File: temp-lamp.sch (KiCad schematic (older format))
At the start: 28 parts, among them P1 USB_5PIN_SHELL, P2 CONN_01X05, P3 CONN_01X08, P4 LED_1, P5 CONN_01X04, SW1 ON/OFF, SW2 RESET, SW3 PGM, U1 MCP73831, U2 ESP-12E, U3 SPX3819M5-3.3, U4 BME280

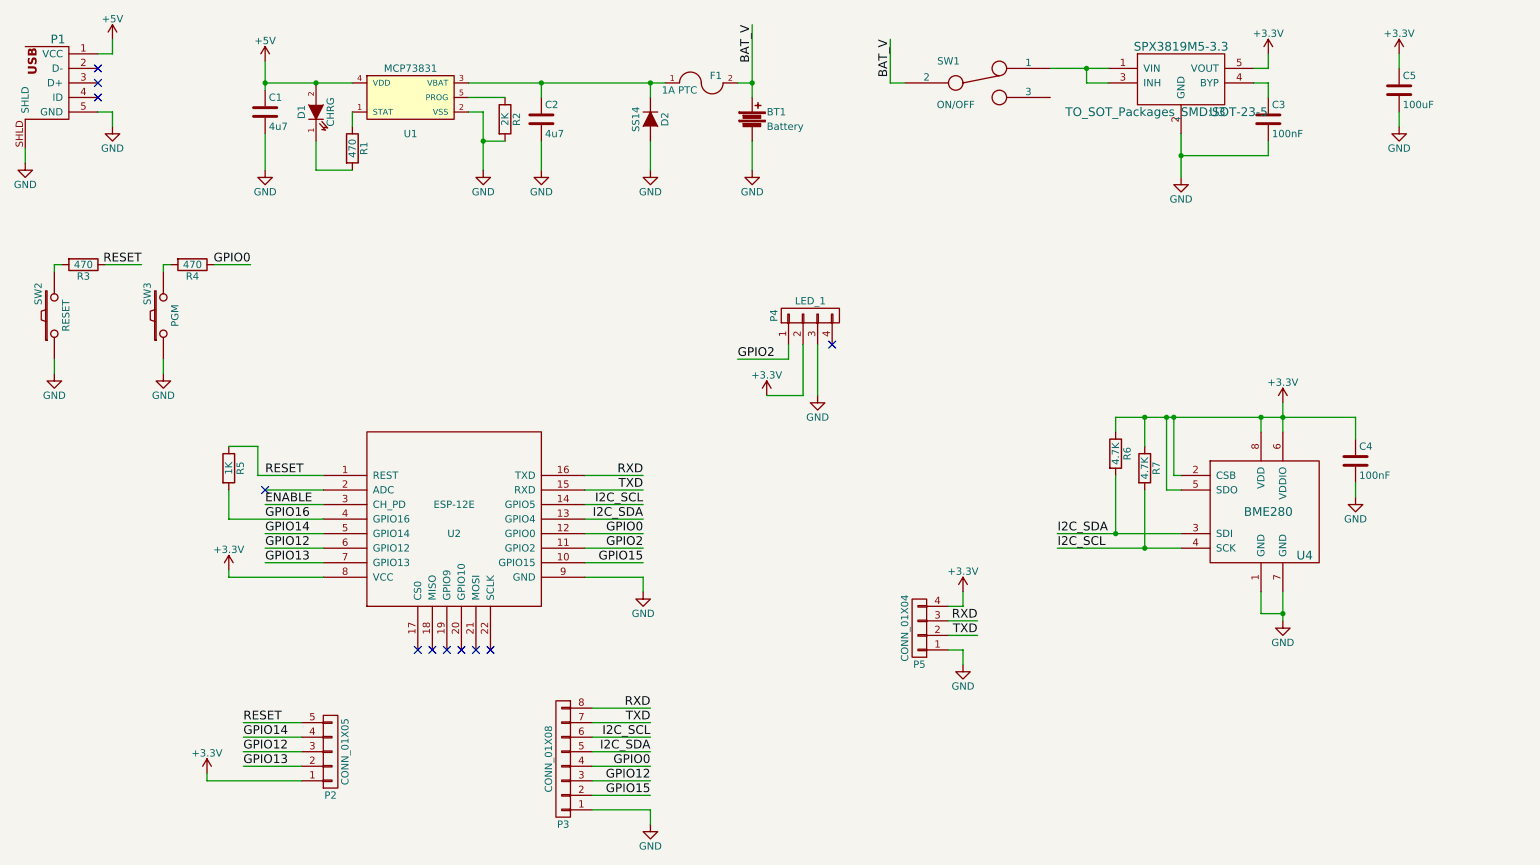
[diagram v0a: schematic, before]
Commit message: Updated pcb.
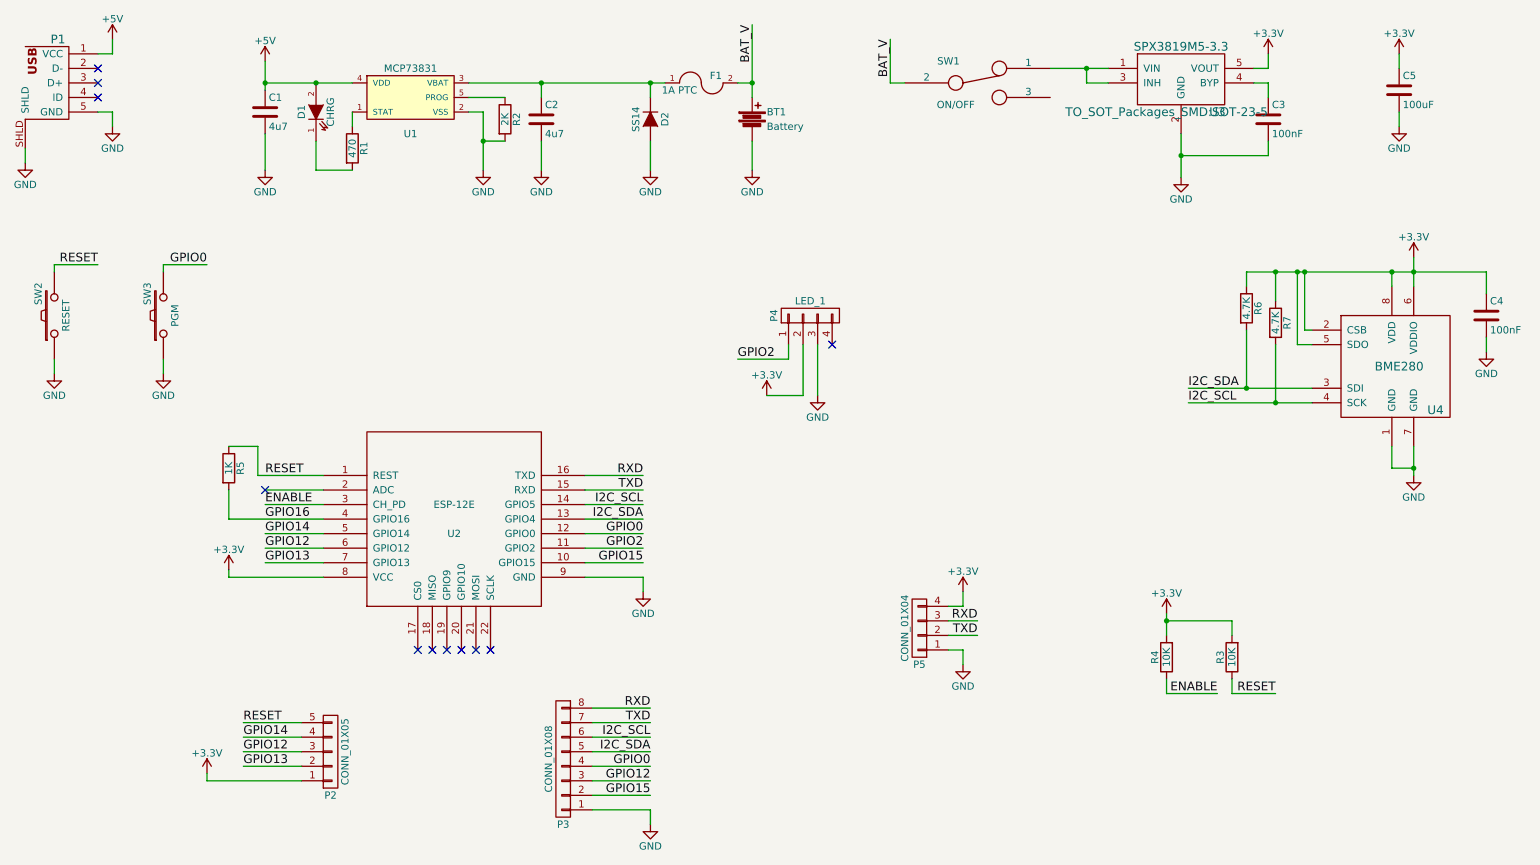
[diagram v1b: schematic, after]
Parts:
- C5: footprint Capacitors_SMD:C_0805_HandSoldering -> Capacitors_SMD:C_1206_HandSoldering
- R3, R4: value 470 -> 10K
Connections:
- net +3V3: now also R3.2, R4.2
- net ENABLE: now also R4.1
- net GPIO0: now also SW3.2; no longer R4.1
- net RESET: now also SW2.2
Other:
- moved on the sheet: C4, R3, R4, R6, R7, U4
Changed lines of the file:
@@
 LIBS:spx3819m5-3
 LIBS:ESP8266
-LIBS:temperature-lamp-cache
+LIBS:temp-lamp-cache
 EELAYER 25 0
 EELAYER END
@@
 	1    0    0    -1
 $EndComp
-$Comp
-L D D2
-U 1 1 5880BBE5
-P 5050 1550
-F 0 "D2" H 5050 1650 50  0000 C CNN
-F 1 "SS14" H 5050 1450 50  0000 C CNN
-F 2 "libs:DIODE_SMA" H 5050 1550 50  0001 C CNN
-F 3 "" H 5050 1550 50  0000 C CNN
-	1    5050 1550
-	0    1    1    0
-$EndComp
 Text Label 5750 900  3    60   ~ 0
 BAT_V
@@
 L BME280 U4
 U 1 1 5880DD6B
-P 9300 4250
-F 0 "U4" H 9550 3950 60  0000 C CNN
-F 1 "BME280" H 9300 4250 60  0000 C CNN
-F 2 "libs:BME280" H 9300 4250 60  0001 C CNN
-F 3 "" H 9300 4250 60  0000 C CNN
-	1    9300 4250
-	1    0    0    -1
-$EndComp
-Wire Wire Line
-	9250 4800 9250 4950
-Wire Wire Line
-	9250 4950 9400 4950
-Wire Wire Line
-	9400 4800 9400 5000
-Connection ~ 9400 4950
+P 10200 3250
+F 0 "U4" H 10450 2950 60  0000 C CNN
+F 1 "BME280" H 10200 3250 60  0000 C CNN
+F 2 "libs:BME280" H 10200 3250 60  0001 C CNN
+F 3 "" H 10200 3250 60  0000 C CNN
+	1    10200 3250
+	1    0    0    -1
+$EndComp
+Wire Wire Line
+	10150 3800 10150 3950
+Wire Wire Line
+	10150 3950 10300 3950
+Wire Wire Line
+	10300 3800 10300 4000
+Connection ~ 10300 3950
 $Comp
 L GND #PWR012
 U 1 1 5880E41C
-P 9400 5000
-F 0 "#PWR012" H 9400 4750 50  0001 C CNN
-F 1 "GND" H 9400 4850 50  0000 C CNN
-F 2 "" H 9400 5000 50  0000 C CNN
-F 3 "" H 9400 5000 50  0000 C CNN
-	1    9400 5000
+P 10300 4000
+F 0 "#PWR012" H 10300 3750 50  0001 C CNN
+F 1 "GND" H 10300 3850 50  0000 C CNN
+F 2 "" H 10300 4000 50  0000 C CNN
+F 3 "" H 10300 4000 50  0000 C CNN
+	1    10300 4000
 	1    0    0    -1
 $EndComp
@@
 L C C4
 U 1 1 5880E8AA
-P 9900 3900
-F 0 "C4" H 9925 4000 50  0000 L CNN
-F 1 "100nF" H 9925 3800 50  0000 L CNN
-F 2 "Capacitors_SMD:C_0603_HandSoldering" H 9938 3750 50  0001 C CNN
-F 3 "" H 9900 3900 50  0000 C CNN
-	1    9900 3900
+P 10800 2900
+F 0 "C4" H 10825 3000 50  0000 L CNN
+F 1 "100nF" H 10825 2800 50  0000 L CNN
+F 2 "Capacitors_SMD:C_0603_HandSoldering" H 10838 2750 50  0001 C CNN
+F 3 "" H 10800 2900 50  0000 C CNN
+	1    10800 2900
 	1    0    0    -1
 $EndComp
@@
 L GND #PWR013
 U 1 1 5880E9DC
-P 9900 4150
-F 0 "#PWR013" H 9900 3900 50  0001 C CNN
-F 1 "GND" H 9900 4000 50  0000 C CNN
-F 2 "" H 9900 4150 50  0000 C CNN
-F 3 "" H 9900 4150 50  0000 C CNN
-	1    9900 4150
-	1    0    0    -1
-$EndComp
-Wire Wire Line
-	9900 4150 9900 4050
+P 10800 3150
+F 0 "#PWR013" H 10800 2900 50  0001 C CNN
+F 1 "GND" H 10800 3000 50  0000 C CNN
+F 2 "" H 10800 3150 50  0000 C CNN
+F 3 "" H 10800 3150 50  0000 C CNN
+	1    10800 3150
+	1    0    0    -1
+$EndComp
+Wire Wire Line
+	10800 3150 10800 3050
 $Comp
 L +3.3V #PWR014
 U 1 1 5880EC60
-P 9400 3500
-F 0 "#PWR014" H 9400 3350 50  0001 C CNN
-F 1 "+3.3V" H 9400 3640 50  0000 C CNN
-F 2 "" H 9400 3500 50  0000 C CNN
-F 3 "" H 9400 3500 50  0000 C CNN
-	1    9400 3500
-	1    0    0    -1
-$EndComp
-Wire Wire Line
-	9900 3600 9900 3750
-Wire Wire Line
-	8250 3600 9900 3600
-Wire Wire Line
-	9400 3500 9400 3700
-Connection ~ 9400 3600
-Wire Wire Line
-	9250 3700 9250 3600
-Wire Wire Line
-	8700 4000 8650 4000
-Wire Wire Line
-	8650 4000 8650 3600
-Connection ~ 9250 3600
-Wire Wire Line
-	8700 4100 8600 4100
-Wire Wire Line
-	8600 4100 8600 3600
-Connection ~ 8650 3600
-Text Label 7850 4400 0    60   ~ 0
+P 10300 2500
+F 0 "#PWR014" H 10300 2350 50  0001 C CNN
+F 1 "+3.3V" H 10300 2640 50  0000 C CNN
+F 2 "" H 10300 2500 50  0000 C CNN
+F 3 "" H 10300 2500 50  0000 C CNN
+	1    10300 2500
+	1    0    0    -1
+$EndComp
+Wire Wire Line
+	10800 2600 10800 2750
+Wire Wire Line
+	9150 2600 10800 2600
+Wire Wire Line
+	10300 2500 10300 2700
+Connection ~ 10300 2600
+Wire Wire Line
+	10150 2700 10150 2600
+Wire Wire Line
+	9600 3000 9550 3000
+Wire Wire Line
+	9550 3000 9550 2600
+Connection ~ 10150 2600
+Wire Wire Line
+	9600 3100 9500 3100
+Wire Wire Line
+	9500 3100 9500 2600
+Connection ~ 9550 2600
+Text Label 8750 3400 0    60   ~ 0
 I2C_SDA
-Text Label 7850 4500 0    60   ~ 0
+Text Label 8750 3500 0    60   ~ 0
 I2C_SCL
 $Comp
 L R R7
 U 1 1 5880F977
-P 8450 3950
-F 0 "R7" V 8530 3950 50  0000 C CNN
-F 1 "4.7K" V 8450 3950 50  0000 C CNN
-F 2 "Resistors_SMD:R_0603_HandSoldering" V 8380 3950 50  0001 C CNN
-F 3 "" H 8450 3950 50  0000 C CNN
-	1    8450 3950
+P 9350 2950
+F 0 "R7" V 9430 2950 50  0000 C CNN
+F 1 "4.7K" V 9350 2950 50  0000 C CNN
+F 2 "Resistors_SMD:R_0603_HandSoldering" V 9280 2950 50  0001 C CNN
+F 3 "" H 9350 2950 50  0000 C CNN
+	1    9350 2950
 	1    0    0    -1
 $EndComp
@@
 L R R6
 U 1 1 5880FB92
-P 8250 3850
-F 0 "R6" V 8330 3850 50  0000 C CNN
-F 1 "4.7K" V 8250 3850 50  0000 C CNN
-F 2 "Resistors_SMD:R_0603_HandSoldering" V 8180 3850 50  0001 C CNN
-F 3 "" H 8250 3850 50  0000 C CNN
-	1    8250 3850
-	1    0    0    -1
-$EndComp
-Wire Wire Line
-	8450 3800 8450 3600
-Connection ~ 8600 3600
-Wire Wire Line
-	8250 3700 8250 3600
-Connection ~ 8450 3600
-Wire Wire Line
-	7850 4500 8700 4500
-Wire Wire Line
-	7850 4400 8700 4400
-Wire Wire Line
-	8450 4100 8450 4500
-Connection ~ 8450 4500
-Wire Wire Line
-	8250 4000 8250 4400
-Connection ~ 8250 4400
+P 9150 2850
+F 0 "R6" V 9230 2850 50  0000 C CNN
+F 1 "4.7K" V 9150 2850 50  0000 C CNN
+F 2 "Resistors_SMD:R_0603_HandSoldering" V 9080 2850 50  0001 C CNN
+F 3 "" H 9150 2850 50  0000 C CNN
+	1    9150 2850
+	1    0    0    -1
+$EndComp
+Wire Wire Line
+	9350 2800 9350 2600
+Connection ~ 9500 2600
+Wire Wire Line
+	9150 2700 9150 2600
+Connection ~ 9350 2600
+Wire Wire Line
+	8750 3500 9600 3500
+Wire Wire Line
+	8750 3400 9600 3400
+Wire Wire Line
+	9350 3100 9350 3500
+Connection ~ 9350 3500
+Wire Wire Line
+	9150 3000 9150 3400
+Connection ~ 9150 3400
 $Comp
 L +3.3V #PWR015
@@
 F 0 "C5" H 10225 1450 50  0000 L CNN
 F 1 "100uF" H 10225 1250 50  0000 L CNN
-F 2 "Capacitors_SMD:C_0805_HandSoldering" H 10238 1200 50  0001 C CNN
+F 2 "Capacitors_SMD:C_1206_HandSoldering" H 10238 1200 50  0001 C CNN
 F 3 "" H 10200 1350 50  0000 C CNN
 	1    10200 1350
@@
 	1    0    0    -1
 $EndComp
-Text Label 1550 2550 2    60   ~ 0
+Text Label 1250 2550 2    60   ~ 0
 RESET
-Text Label 2300 2550 2    60   ~ 0
+Text Label 2000 2550 2    60   ~ 0
 GPIO0
 Wire Wire Line
 	950  2600 950  2550
 Wire Wire Line
-	950  2550 1000 2550
+	950  2550 1250 2550
 Wire Wire Line
 	1700 2600 1700 2550
 Wire Wire Line
-	1700 2550 1750 2550
+	1700 2550 2000 2550
 Wire Wire Line
 	1700 3300 1700 3200
@@
 L R R4
 U 1 1 58815A9F
-P 1900 2550
-F 0 "R4" V 1980 2550 50  0000 C CNN
-F 1 "470" V 1900 2550 50  0000 C CNN
-F 2 "Resistors_SMD:R_0603_HandSoldering" V 1830 2550 50  0001 C CNN
-F 3 "" H 1900 2550 50  0000 C CNN
-	1    1900 2550
-	0    1    1    0
+P 8600 5250
+F 0 "R4" V 8680 5250 50  0000 C CNN
+F 1 "10K" V 8600 5250 50  0000 C CNN
+F 2 "Resistors_SMD:R_0603_HandSoldering" V 8530 5250 50  0001 C CNN
+F 3 "" H 8600 5250 50  0000 C CNN
+	1    8600 5250
+	-1   0    0    1
 $EndComp
 $Comp
 L R R3
 U 1 1 58815ECD
-P 1150 2550
-F 0 "R3" V 1230 2550 50  0000 C CNN
-F 1 "470" V 1150 2550 50  0000 C CNN
-F 2 "Resistors_SMD:R_0603_HandSoldering" V 1080 2550 50  0001 C CNN
-F 3 "" H 1150 2550 50  0000 C CNN
-	1    1150 2550
-	0    1    1    0
-$EndComp
-Wire Wire Line
-	1300 2550 1550 2550
-Wire Wire Line
-	2050 2550 2300 2550
+P 9050 5250
+F 0 "R3" V 9130 5250 50  0000 C CNN
+F 1 "10K" V 9050 5250 50  0000 C CNN
+F 2 "Resistors_SMD:R_0603_HandSoldering" V 8980 5250 50  0001 C CNN
+F 3 "" H 9050 5250 50  0000 C CNN
+	1    9050 5250
+	-1   0    0    1
+$EndComp
 $Comp
 L CONN_01X05 P2
@@
 Wire Wire Line
 	7300 5100 7100 5100
+Text Label 8950 5500 2    60   ~ 0
+ENABLE
+$Comp
+L +3.3V #PWR027
+U 1 1 58A46612
+P 8600 4950
+F 0 "#PWR027" H 8600 4800 50  0001 C CNN
+F 1 "+3.3V" H 8600 5090 50  0000 C CNN
+F 2 "" H 8600 4950 50  0000 C CNN
+F 3 "" H 8600 4950 50  0000 C CNN
+	1    8600 4950
+	1    0    0    -1
+$EndComp
+Wire Wire Line
+	8600 5400 8600 5500
+Wire Wire Line
+	8600 5500 8950 5500
+Wire Wire Line
+	9050 5100 9050 5000
+Wire Wire Line
+	9050 5000 8600 5000
+Wire Wire Line
+	8600 4950 8600 5100
+Connection ~ 8600 5000
+Text Label 9350 5500 2    60   ~ 0
+RESET
+Wire Wire Line
+	9050 5400 9050 5500
+Wire Wire Line
+	9050 5500 9350 5500
+$Comp
+L D D2
+U 1 1 58AAD489
+P 5050 1550
+F 0 "D2" H 5050 1650 50  0000 C CNN
+F 1 "SS14" H 5050 1450 50  0000 C CNN
+F 2 "libs:DIODE_SMA" H 5050 1550 50  0001 C CNN
+F 3 "" H 5050 1550 50  0000 C CNN
+	1    5050 1550
+	0    1    1    0
+$EndComp
 $EndSCHEMATC
